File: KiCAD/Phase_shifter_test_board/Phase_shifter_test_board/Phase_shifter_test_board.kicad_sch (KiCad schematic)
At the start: 7 parts, among them J3 Conn_01x10_Pin

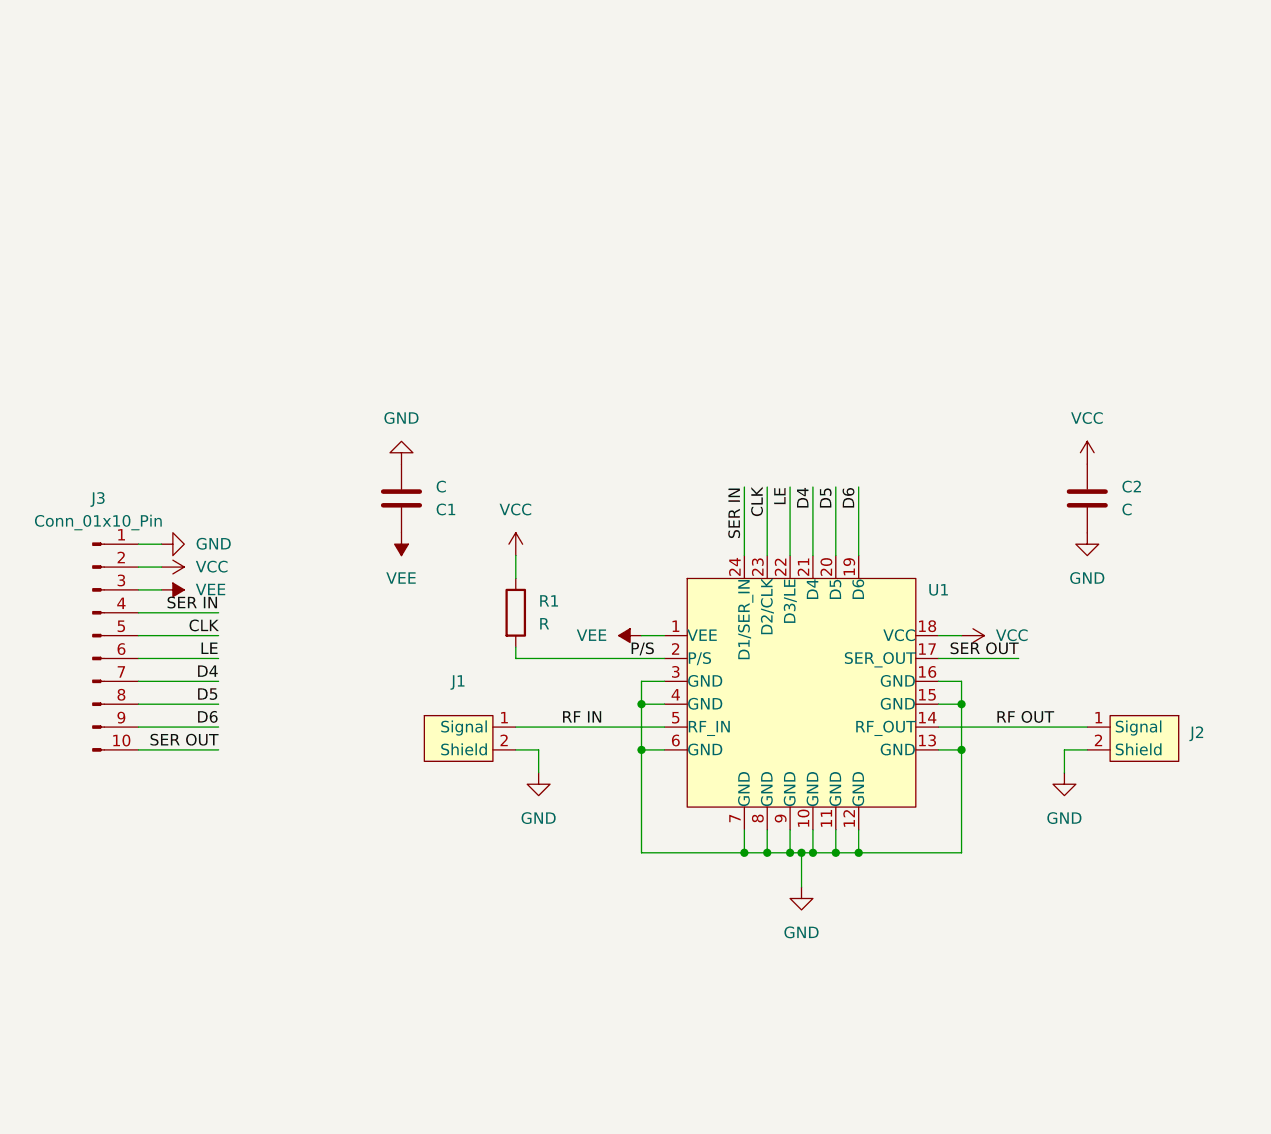
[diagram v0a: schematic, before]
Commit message: phase shifter
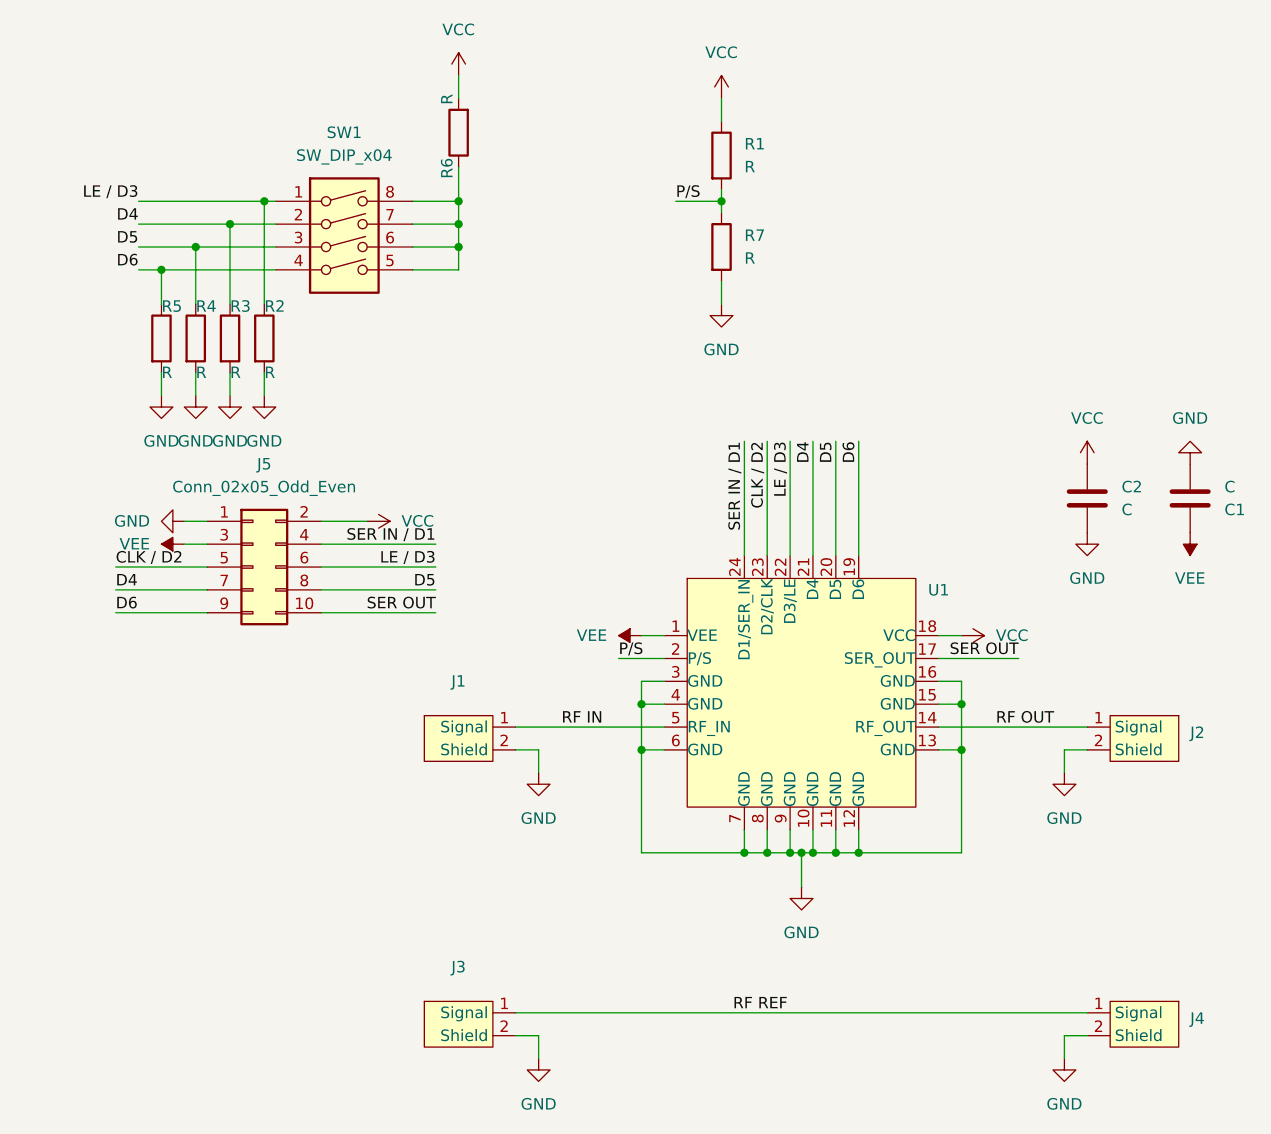
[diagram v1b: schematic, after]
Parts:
- removed J3: Conn_01x10_Pin, Connector_PinHeader_2.54mm:PinHeader_1x10_P2.54mm_Vertical_SMD_Pin1Left, symbol Connector:Conn_01x10_Pin
- added J3, J4: ~, Phase_shifter:Conn, symbol Phase_shifter:RF-conn
- added J5: Conn_02x05_Odd_Even, Connector_PinHeader_2.54mm:PinHeader_2x05_P2.54mm_Vertical, symbol Connector_Generic:Conn_02x05_Odd_Even
- added R2, R3, R4, R5, R6, R7: R, Resistor_SMD:R_0603_1608Metric_Pad0.98x0.95mm_HandSolder, symbol Device:R
- added SW1: SW_DIP_x04, Button_Switch_THT:SW_DIP_SPSTx04_Slide_9.78x12.34mm_W7.62mm_P2.54mm, symbol Switch:SW_DIP_x04
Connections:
- net D4: now also J5.7 (Pin_7), R3.1, SW1.2
- net D5: now also J5.8 (Pin_8), R4.1, SW1.3
- net D6: now also J5.9 (Pin_9), R5.1, SW1.4
- net GND: now also J3.2 (Shield), J4.2 (Shield), J5.1 (Pin_1), R2.2, R3.2, R4.2, R5.2, R7.2
- net P/S: now also R7.1
- net SER OUT: now also J5.10 (Pin_10)
- net VCC: now also J5.2 (Pin_2), R6.2
- net VEE: now also J5.3 (Pin_3)
- net CLK renamed CLK / D2
- net CLK / D2: now also J5.5 (Pin_5)
- net LE renamed LE / D3
- net LE / D3: now also J5.6 (Pin_6), R2.1, SW1.1
- net SER IN renamed SER IN / D1
- net SER IN / D1: now also J5.4 (Pin_4)
- new net: R6.1, SW1.5, SW1.6, SW1.7, SW1.8
- new net RF REF: J3.1 (Signal), J4.1 (Signal)
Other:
- moved on the sheet: C1, R1
